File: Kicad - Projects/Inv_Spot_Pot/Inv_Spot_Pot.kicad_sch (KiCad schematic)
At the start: 71 parts, among them J1 Screw_Terminal_01x03, J2 PWM, J3 Display_Power, J4 Current_Sense, J5 ThSw, Q1 40T120, Q2 40T120, Q3 40T120, Q4 40T120, T1 Transformer_1P_1S, U2 LTV-817S, U3 TL431DBZ

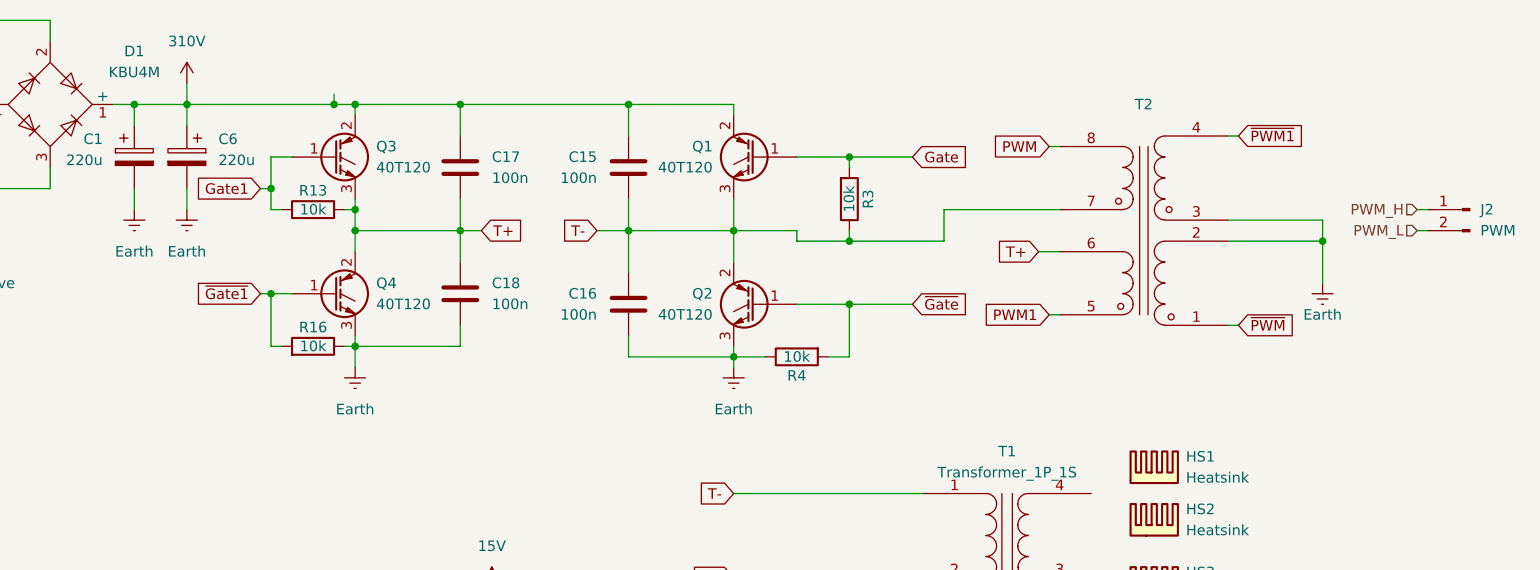
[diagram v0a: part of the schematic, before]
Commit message: Ajustes Finais
Ajustes Finais do código, esquemáticos e layouts

Ainda faltam ajustes finos
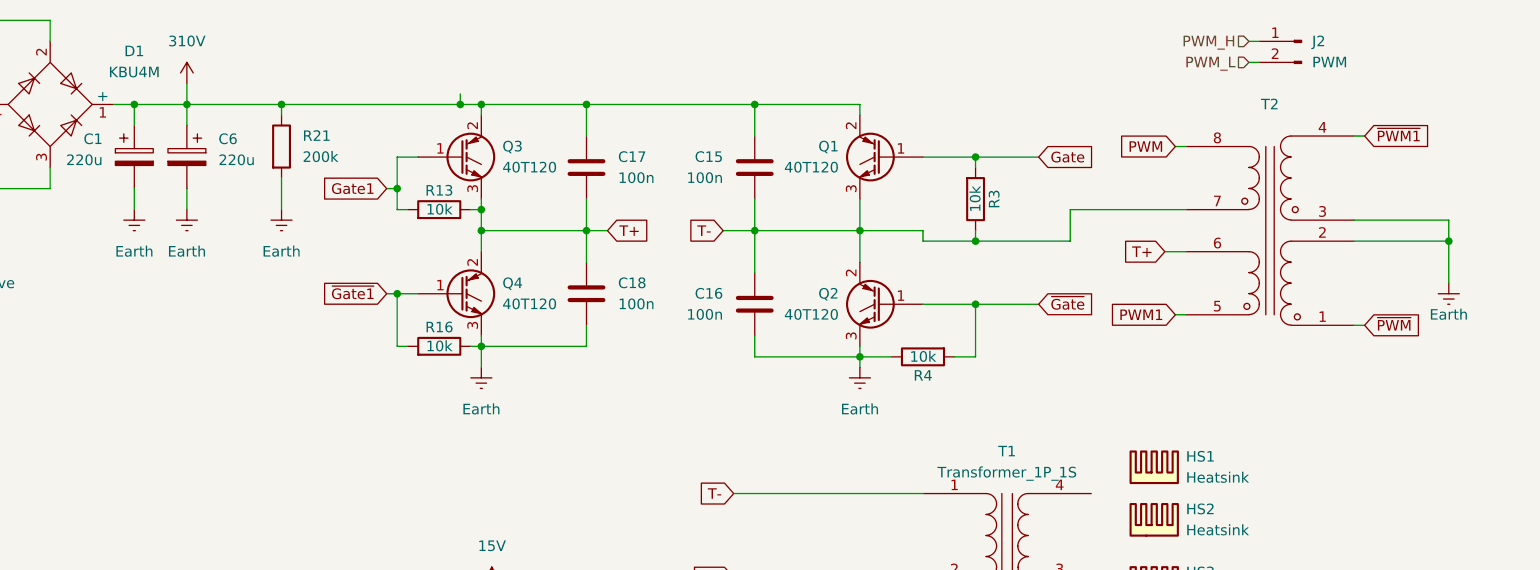
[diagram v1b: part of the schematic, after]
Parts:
- added R21: 200k, Resistor_SMD:R_1206_3216Metric_Pad1.30x1.75mm_HandSolder, symbol Device:R
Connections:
- net 310V: now also R21.1
- net Earth: now also R21.2
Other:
- moved on the sheet: C15, C16, C17, C18, J2, Q1, Q2, Q3, Q4, R13, R16, R3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
